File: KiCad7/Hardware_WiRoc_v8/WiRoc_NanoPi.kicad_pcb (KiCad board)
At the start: 6 copper layers, 97.7 x 68.7 mm, 202 parts, among them J1 Conn_02x05_Odd_Even, J10 Conn_01x09_Socket, J2 Conn_01x04, J3 Micro_SD_Card_Det1, J4 Conn_01x09_Socket, J5 Conn_01x04_Socket, J6 HAT_Conn_DBG, J8 Conn_01x06, J9 Conn_Coaxial, Q1 L2N7002WT1G, SW1 SW_SPST, U1 DRF1268DS, U13 SGM803-RXN3L, U14 KLM8G1WEPD-B031, U15 RT8059, U16 RT8059, U17 RT8059, U18 MP2143DJ, U2 OLED, U3 AXP209, U4 74LS73, U5 SY6280, U6 BatteryPadM, U7 BatteryPadP, U8 SP3232ECY-L, U9 PCF8563T, Y1 32.768kHz, Y2 24MHz/18pF

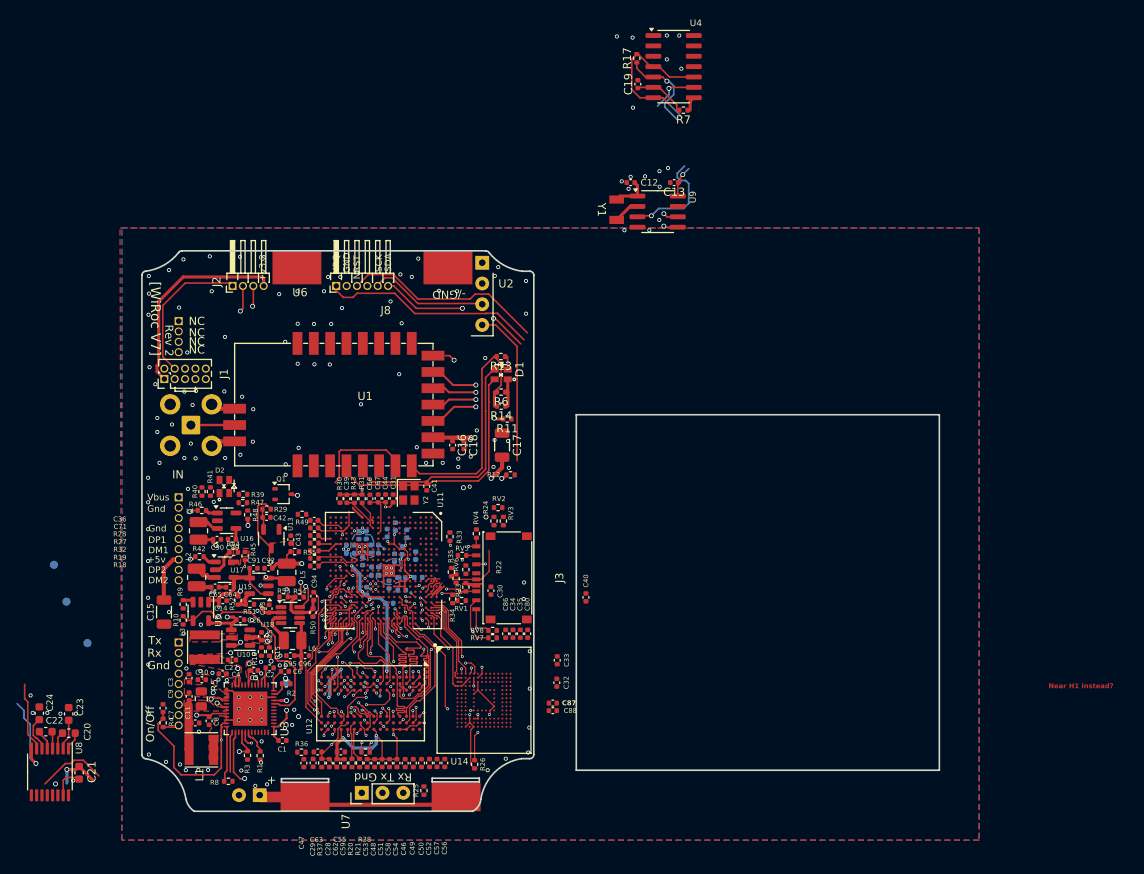
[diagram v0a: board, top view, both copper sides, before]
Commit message: more routing of v8
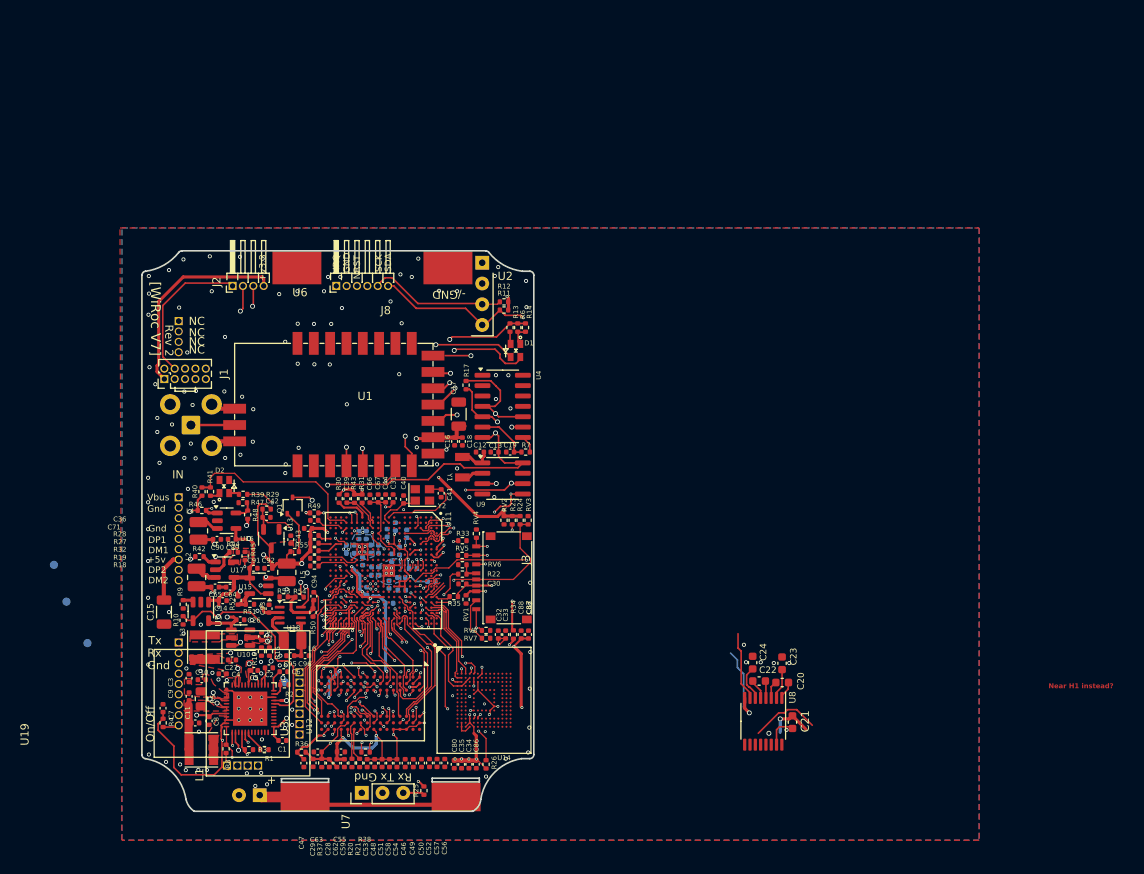
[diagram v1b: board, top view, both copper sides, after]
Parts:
- added U19: ESP32-C6-Board, WiRoc:ESP32Hosted-C6-Board, F.Cu at (56.3, 102.2)
- U18: footprint Package_TO_SOT_SMD:TSOT-23-8 -> WiRoc:TSOT-23-8-Thinner-Pads
- moved C20 87.6 mm to (124.9, 99.7)
- moved C21 87.6 mm to (126.2, 104.5)
- moved C22 87.6 mm to (122.1, 99.5)
- moved C23 87.6 mm to (124.9, 97.3)
- moved C24 87.6 mm to (121.3, 97.2)
- moved U8 87.6 mm to (122.6, 104.4)
- moved C19 47.7 mm to (91.6, 71.5), turned to 180 degrees
- moved U4 46.6 mm to (90.7, 65.8)
- moved R7 46.1 mm to (93.5, 71.5)
- moved R17 45.2 mm to (86.2, 63.2)
- moved C13 39.7 mm to (89.7, 71.5)
- moved C12 37.8 mm to (87.9, 71.5)
- moved U9 37.8 mm to (90.7, 74.7)
- moved Y1 36.8 mm to (85.8, 73.3)
- moved C40 25.4 mm to (78.5, 77.2)
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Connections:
- U11 pad L18: unconnected-(U11D-PD16/MDC-PadL18) -> WIFI-DataReady
- U11 pad L19: unconnected-(U11D-PD17/MDIO-PadL19) -> WIFI-HandShake
- U14 pad M6: eMMC-CMD -> eMMC-CLK
- U14 pad P2: unconnected-(U14-NC102-PadP2) -> GND
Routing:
- net VDD_SYS_3.3V: track 182.5 -> 298.9 mm, vias 19 -> 29
- net SDA: track 40.9 -> 125.5 mm, vias 2 -> 5
- net SCK: track 33.2 -> 111.1 mm, vias 3 -> 4
- net IRQ: track 6.87 -> 77.2 mm, vias 0 -> 2
- net N_OE: track 13.2 -> 76.3 mm
- net LDO1: track 35.4 -> 82.2 mm, vias 3 -> 5
- net UART0_TX: track 0.00 -> 40.3 mm, vias 0 -> 1
- net USBHost-DP2: track 0.00 -> 39.9 mm, vias 0 -> 1
- net USBHost-DM2: track 0.00 -> 38.6 mm, vias 0 -> 1
- net USBHost-DP1: track 0.00 -> 37.4 mm, vias 0 -> 1
- net USBHost-DM1: track 0.00 -> 37.2 mm, vias 0 -> 1
- net  GPIOA10/STATUS-LED: track 0.00 -> 35.6 mm, vias 0 -> 2
- net Net-(U11D-PA5/UART0_RX/PWM0/PA_EINT5): track 0.00 -> 33.8 mm, vias 0 -> 2
- net GPIOL8/PWR-STB: track 4.75 -> 38.1 mm, vias 1 -> 3
- net VDD_5V: track 42.3 -> 69.6 mm
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- added copper zone on In4.Cu, net VDD_SYS_3.3V
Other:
- board size 97.7 x 68.7 mm -> 48 x 68.7 mm
